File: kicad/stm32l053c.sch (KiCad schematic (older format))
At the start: 52 parts, among them J1 Water_Level, J2 Motion, J3 Door, J4 Door_Led, J5 AIN3, J6 Pump, J7 BATTERY, P1 SWD, Q1 Q_NMOS_GSD, U1 MCP1703A-5002_SOT223, U2 STM32L053C8_LQFP48, U3 ADS1015, U4 UFL_SMA, U5 RFM92/95, U6 MCP1703A-3302_SOT223

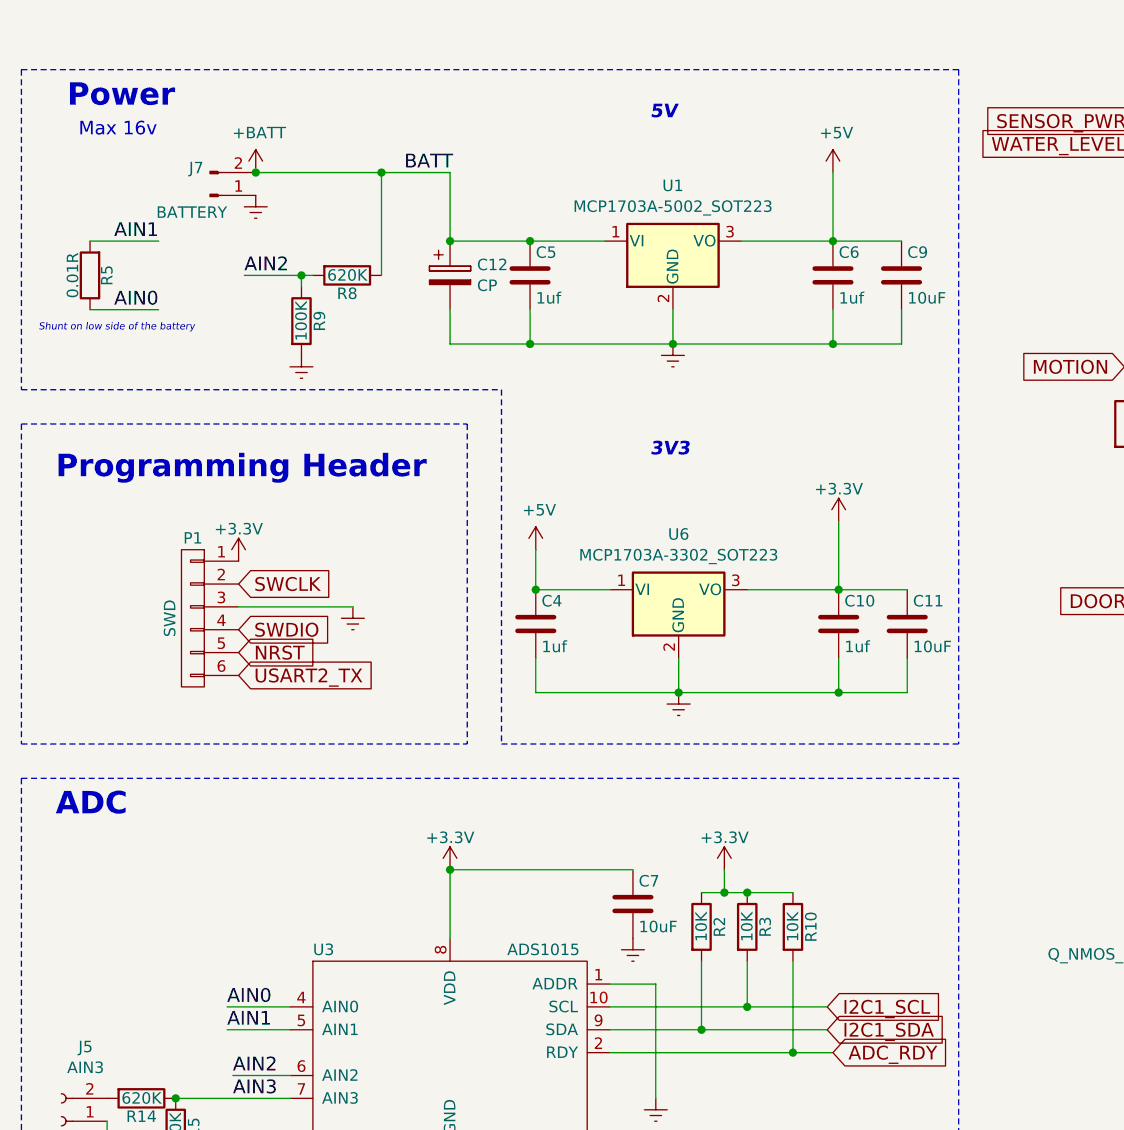
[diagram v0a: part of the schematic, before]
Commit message: Protection
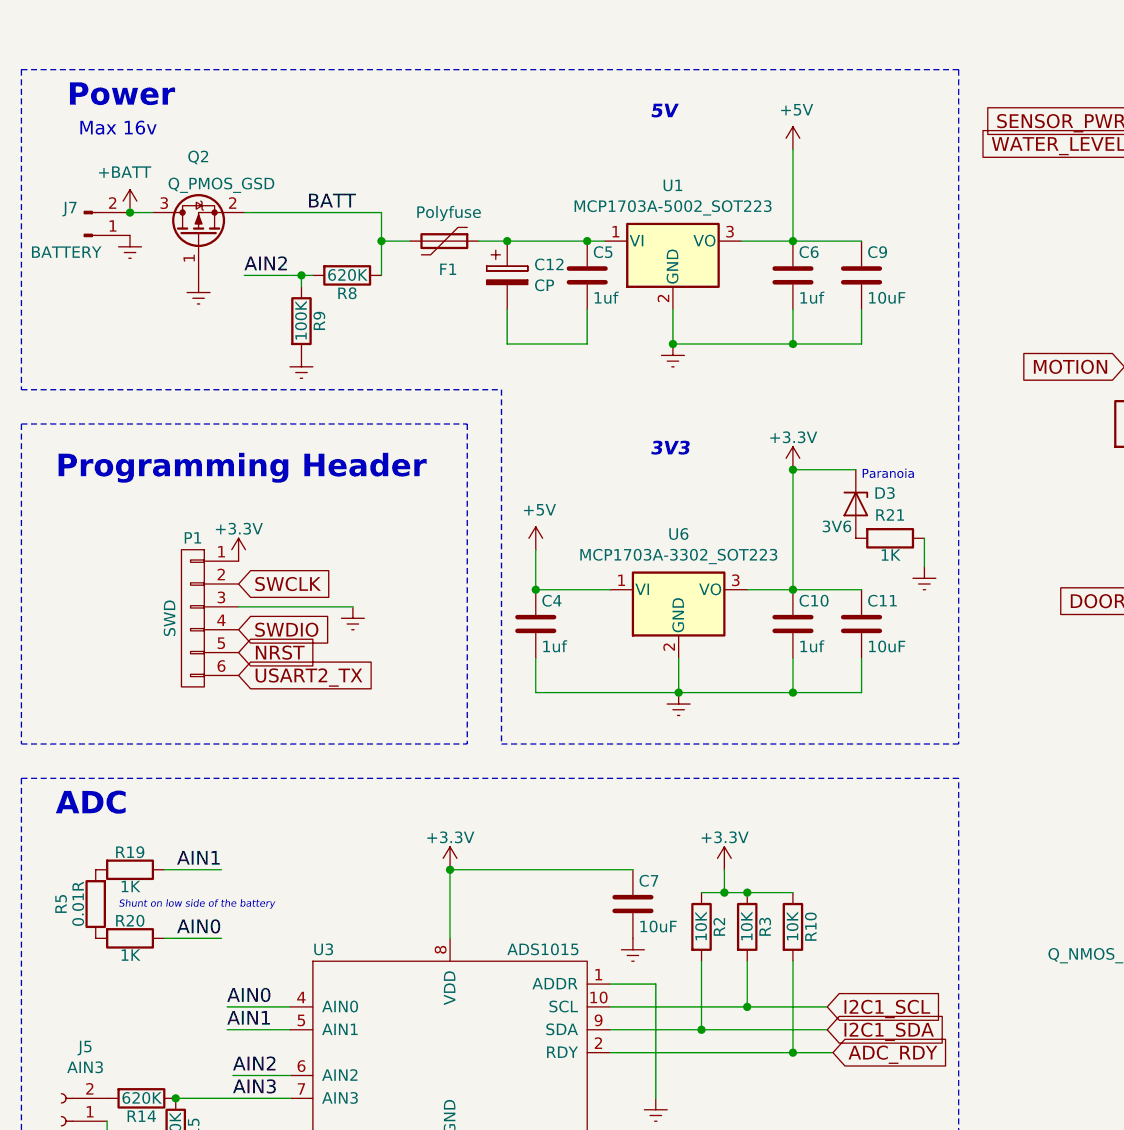
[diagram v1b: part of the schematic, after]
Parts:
- added D3: 3V6, Diode_THT:D_T-1_P5.08mm_Horizontal, symbol Device:D_Zener
- added F1: Polyfuse, Resistor_SMD:R_1812_4532Metric_Pad1.30x3.40mm_HandSolder, symbol Device:Polyfuse
- added Q2: Q_PMOS_GSD, Package_TO_SOT_SMD:SOT-23_Handsoldering, symbol Device:Q_PMOS_GSD
- added R19, R20, R21: 1K, Resistor_SMD:R_0603_1608Metric_Pad1.05x0.95mm_HandSolder, symbol Device:R
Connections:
- net +3V3: now also D3.1 (K)
- net +BATT: now also Q2.3 (D); no longer C12.1, C5.1, R8.1, U1.1 (VI)
- net AIN0: now also R20.1; no longer R5.1
- net AIN1: now also R19.1; no longer R5.2
- net Earth: now also Q2.1 (G), R21.1; no longer C12.2, C5.2
- new net: C12.1, C5.1, F1.1, U1.1 (VI)
- new net: C12.2, C5.2
- new net: R20.2, R5.1
- new net: R19.2, R5.2
- new net: D3.2 (A), R21.2
- new net BATT: F1.2, Q2.2 (S), R8.1
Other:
- note added: "Paranoia"
- moved on the sheet: C10, C11, C12, C5, C6, C9, J7, R5
